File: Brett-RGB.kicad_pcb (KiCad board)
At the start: 2 copper layers, 223 x 71 mm, 182 parts, among them P1 CONN_02X05, P2 USB_OTG, SW1 SW_PUSH, SW10 SW_PUSH, SW11 SW_PUSH, SW12 SW_PUSH, SW13 SW_PUSH, SW14 SW_PUSH, SW15 SW_PUSH, SW16 SW_PUSH, SW17 SW_PUSH, SW18 SW_PUSH, SW19 SW_PUSH, SW2 SW_PUSH, SW20 SW_PUSH, SW21 SW_PUSH, SW22 SW_PUSH, SW23 SW_PUSH, SW24 SW_PUSH, SW25 SW_PUSH, SW26 SW_PUSH, SW27 SW_PUSH, SW28 SW_PUSH, SW29 SW_PUSH, SW3 SW_PUSH, SW30 SW_PUSH, SW31 SW_PUSH, SW32 SW_PUSH, SW33 SW_PUSH, SW34 SW_PUSH, SW35 SW_PUSH, SW36 SW_PUSH, SW37 SW_PUSH, SW38 SW_PUSH, SW39 SW_PUSH, SW4 SW_PUSH, SW40 SW_PUSH, SW41 SW_PUSH, SW42 SW_PUSH, SW43 SW_PUSH, SW44 SW_PUSH, SW45 SW_PUSH, SW46 SW_PUSH, SW47 SW_PUSH, SW48 Reset, SW5 SW_PUSH, SW6 SW_PUSH, SW7 SW_PUSH, SW8 SW_PUSH, SW9 SW_PUSH, U1 IS31FL3732, U2 MK20DX256VLH7, X1 CRYSTAL_SMD

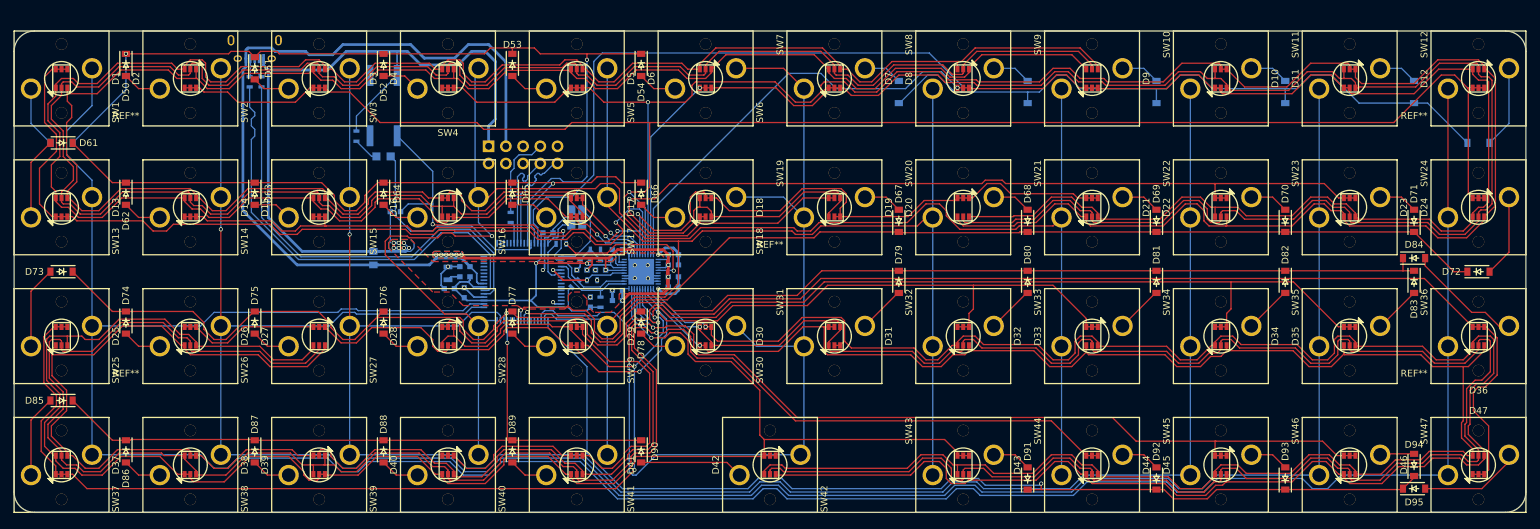
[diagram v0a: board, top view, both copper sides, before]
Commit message: Reworked the Board
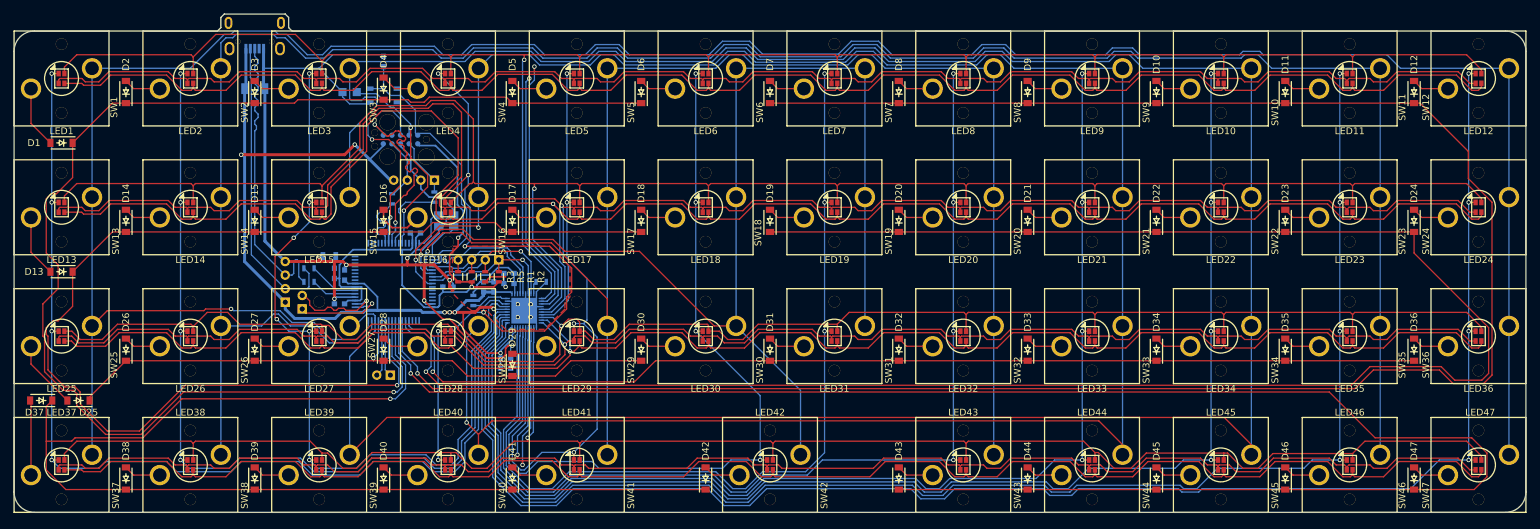
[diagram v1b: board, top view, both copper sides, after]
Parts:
- removed C14, C15, C17, C20, C21: 0.1uF, Capacitors_SMD:C_0603
- removed C18, C19: 1uF, Capacitors_SMD:C_0603
- removed D48: LED, LEDs:LED_0805
- removed D49, D50, D51, D52, D53, D54, D55, D56, D57, D58, D59, D60, D61, D62, D63, D64, D65, D66, D67, D68, D69, D70, D71, D72, D73, D74, D75, D76, D77, D78, D79, D80, D81, D82, D83, D84, D85, D86, D87, D88, D89, D90, D91, D92, D93, D94, D95: D_Small, Diodes_SMD:SOD-123
- added C11: 0.1uF, Capacitors_SMD:C_0603, B.Cu at (97.2, 64.8)
- added LED1: Led_RGB_CA, lib.pretty:RGB-0606, F.Cu at (45.0, 42.0)
- added LED10: Led_RGB_CA, lib.pretty:RGB-0606, F.Cu at (216.0, 42.0)
- added LED11: Led_RGB_CA, lib.pretty:RGB-0606, F.Cu at (235.0, 42.0)
- added LED12: Led_RGB_CA, lib.pretty:RGB-0606, F.Cu at (254.0, 42.0)
- added LED13: Led_RGB_CA, lib.pretty:RGB-0606, F.Cu at (45.0, 61.0)
- added LED14: Led_RGB_CA, lib.pretty:RGB-0606, F.Cu at (64.0, 61.0)
- added LED15: Led_RGB_CA, lib.pretty:RGB-0606, F.Cu at (83.0, 61.0)
- added LED16: Led_RGB_CA, lib.pretty:RGB-0606, F.Cu at (102.0, 61.0)
- added LED17: Led_RGB_CA, lib.pretty:RGB-0606, F.Cu at (121.0, 61.0)
- added LED18: Led_RGB_CA, lib.pretty:RGB-0606, F.Cu at (140.0, 61.0)
- added LED19: Led_RGB_CA, lib.pretty:RGB-0606, F.Cu at (159.0, 61.0)
- added LED2: Led_RGB_CA, lib.pretty:RGB-0606, F.Cu at (64.0, 42.0)
- added LED20: Led_RGB_CA, lib.pretty:RGB-0606, F.Cu at (178.0, 61.0)
- added LED21: Led_RGB_CA, lib.pretty:RGB-0606, F.Cu at (197.0, 61.0)
- added LED22: Led_RGB_CA, lib.pretty:RGB-0606, F.Cu at (216.0, 61.0)
- added LED23: Led_RGB_CA, lib.pretty:RGB-0606, F.Cu at (235.0, 61.0)
- added LED24: Led_RGB_CA, lib.pretty:RGB-0606, F.Cu at (254.0, 61.0)
- added LED25: Led_RGB_CA, lib.pretty:RGB-0606, F.Cu at (45.0, 80.0)
- added LED26: Led_RGB_CA, lib.pretty:RGB-0606, F.Cu at (64.0, 80.0)
- added LED27: Led_RGB_CA, lib.pretty:RGB-0606, F.Cu at (83.0, 80.0)
- added LED28: Led_RGB_CA, lib.pretty:RGB-0606, F.Cu at (102.0, 80.0)
- added LED29: Led_RGB_CA, lib.pretty:RGB-0606, F.Cu at (121.0, 80.0)
- added LED3: Led_RGB_CA, lib.pretty:RGB-0606, F.Cu at (83.0, 42.0)
- added LED30: Led_RGB_CA, lib.pretty:RGB-0606, F.Cu at (140.0, 80.0)
- added LED31: Led_RGB_CA, lib.pretty:RGB-0606, F.Cu at (159.0, 80.0)
- added LED32: Led_RGB_CA, lib.pretty:RGB-0606, F.Cu at (178.0, 80.0)
- added LED33: Led_RGB_CA, lib.pretty:RGB-0606, F.Cu at (197.0, 80.0)
- added LED34: Led_RGB_CA, lib.pretty:RGB-0606, F.Cu at (216.0, 80.0)
- added LED35: Led_RGB_CA, lib.pretty:RGB-0606, F.Cu at (235.0, 80.0)
- added LED36: Led_RGB_CA, lib.pretty:RGB-0606, F.Cu at (254.0, 80.0)
- added LED37: Led_RGB_CA, lib.pretty:RGB-0606, F.Cu at (45.0, 99.0)
- added LED38: Led_RGB_CA, lib.pretty:RGB-0606, F.Cu at (64.0, 99.0)
- added LED39: Led_RGB_CA, lib.pretty:RGB-0606, F.Cu at (83.0, 99.0)
- added LED4: Led_RGB_CA, lib.pretty:RGB-0606, F.Cu at (102.0, 42.0)
- added LED40: Led_RGB_CA, lib.pretty:RGB-0606, F.Cu at (102.0, 99.0)
- added LED41: Led_RGB_CA, lib.pretty:RGB-0606, F.Cu at (121.0, 99.0)
- added LED42: Led_RGB_CA, lib.pretty:RGB-0606, F.Cu at (149.5, 99.0)
- added LED43: Led_RGB_CA, lib.pretty:RGB-0606, F.Cu at (178.0, 99.0)
- added LED44: Led_RGB_CA, lib.pretty:RGB-0606, F.Cu at (197.0, 99.0)
- added LED45: Led_RGB_CA, lib.pretty:RGB-0606, F.Cu at (216.0, 99.0)
- added LED46: Led_RGB_CA, lib.pretty:RGB-0606, F.Cu at (235.0, 99.0)
- added LED47: Led_RGB_CA, lib.pretty:RGB-0606, F.Cu at (254.0, 99.0)
- added LED48: LED, lib.pretty:LED_0805, B.Cu at (87.5, 44.0)
- added LED5: Led_RGB_CA, lib.pretty:RGB-0606, F.Cu at (121.0, 42.0)
- added LED6: Led_RGB_CA, lib.pretty:RGB-0606, F.Cu at (140.0, 42.0)
- added LED7: Led_RGB_CA, lib.pretty:RGB-0606, F.Cu at (159.0, 42.0)
- added LED8: Led_RGB_CA, lib.pretty:RGB-0606, F.Cu at (178.0, 42.0)
- added LED9: Led_RGB_CA, lib.pretty:RGB-0606, F.Cu at (197.0, 42.0)
- added P3: CONN_01X04, lib.pretty:Conn-4, B.Cu at (97.0, 57.0)
- added P4: FLASH_HDR, lib.pretty:JLINK_NEEDLE, B.Cu at (95.0, 51.0)
- added P5: CONN_01X04, lib.pretty:Conn-4, B.Cu at (106.5, 68.8)
- added P6: CONN_01X02, lib.pretty:Conn-2, B.Cu at (92.5, 85.8)
- added P7: CONN_01X02, lib.pretty:Conn-2, B.Cu at (80.5, 75.0)
- added R11: 100, Resistors_SMD:R_0603, B.Cu at (100.0, 59.5)
- C1: value 100uF -> 0.1uF; footprint Capacitors_SMD:C_0805 -> Capacitors_SMD:C_0603
- C12: value 100n -> 0.1uF
- C13, C3: value 1uF -> 0.1uF
- C4: value 0.1uF -> 100uF; footprint Capacitors_SMD:C_0603 -> Capacitors_SMD:C_1206
- C5, C7: value 0.1uF -> 1uF
- C9: value 2.2uF -> 0.1uF
- D1, D10, D11, D12, D13, D14, D15, D16, D17, D18, D19, D2, D20, D21, D22, D23, D24, D25, D26, D27, D28, D29, D3, D30, D31, D32, D33, D34, D35, D36, D37, D38, D39, D4, D40, D41, D42, D43, D44, D45, D46, D47, D5, D6, D7, D8, D9: value LED_RGB -> D_Small; footprint mx2a:plcc-6 -> lib.pretty:SOD-123
- P1: value CONN_02X05 -> USB_OTG; footprint Pin_Headers:Pin_Header_Straight_2x05 -> lib.pretty:Micro-USB_629105150521
- P2: value USB_OTG -> CONN_01X04; footprint Connect:USB_Micro-B -> lib.pretty:Conn-4
- R1: value 1k -> 100k; moved to F.Cu
- R2: moved to F.Cu
- R3: value 33 -> 4.7k; moved to F.Cu
- R4: value 33 -> 100k
- R5: value 5M -> 4.7k; footprint Resistors_SMD:R_0805 -> Resistors_SMD:R_0603; moved to F.Cu
- R6: value 20k -> 33
- R7: value 1k -> 33
- R8: value 1k -> 20k
- R9: value 100k -> 5M; footprint Resistors_SMD:R_0603 -> Resistors_SMD:R_0805
- SW1, SW10, SW11, SW12, SW13, SW14, SW15, SW16, SW17, SW18, SW19, SW2, SW20, SW21, SW22, SW23, SW24, SW25, SW26, SW27, SW28, SW29, SW3, SW30, SW31, SW32, SW33, SW34, SW35, SW36, SW37, SW38, SW39, SW4, SW40, SW41, SW42, SW43, SW44, SW45, SW46, SW47, SW5, SW6, SW7, SW8, SW9: footprint mx2a:RomerG -> lib.pretty:RomerG
- SW48: value Reset -> TAC_SWITCH; footprint mx2a:KSEM31GLFS -> lib.pretty:PTS810
- U1: value IS31FL3732 -> IS31FL3737
- U2: value MK20DX256VLH7 -> MK20DX256VLH7-RESCUE-RainbowFox
- moved C4 66.4 mm to (73.5, 43.5)
- moved R4 50.7 mm to (115.8, 72.0), turned to 180 degrees
- moved R6 42.3 mm to (81.5, 70.0), turned to 180 degrees
- moved R3 42.1 mm to (103.5, 71.2), turned to 90 degrees
- moved P1 39.9 mm to (73.5, 32.0), turned to 0 degrees
- moved R7 39.3 mm to (81.5, 72.0), turned to 180 degrees
- moved R9 38.9 mm to (84.5, 68.2)
- moved P2 34.8 mm to (78.0, 72.0), turned to 90 degrees
- moved R1 28.1 mm to (107.5, 71.2)
- moved C5 28.0 mm to (107.2, 72.8), turned to 90 degrees
- moved C3 26.5 mm to (108.8, 72.8), turned to 90 degrees
- moved C13 25.1 mm to (102.0, 72.8), turned to 0 degrees
- moved C2 24.4 mm to (111.0, 72.2), turned to 180 degrees
- moved C12 22.2 mm to (92.5, 39.5), turned to 90 degrees
- moved C1 20.1 mm to (111.0, 70.8), turned to 180 degrees
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- renumbered REF** to ?
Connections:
- net /MCU/X+ renamed Net-(U2-Pad32)
- net /MCU/X- renamed Net-(U2-Pad33)
- C1 pad 1: GND -> +3V3
- C1 pad 2: +5V -> GND
- C10 pad 1: GND -> +5V
- C10 pad 2: +5V -> GND
- C13 pad 1: +5V -> +3V3
- C2 pad 1: +5V -> +3V3
- C6 pad 1: +3V3 -> +5V
- C7 pad 1: +3V3 -> +5V
- C8 pad 2: GND -> Net-(C8-Pad2)
- C9 pad 1: Net-(C9-Pad1) -> +3V3
- C9 pad 2: +3V3 -> GND
- D1 pad 1: /MCU/A1 -> /MCU/PTD0
- D1 pad 2: /MCU/A2 -> Net-(D1-Pad2)
- D10 pad 1: /MCU/A9 -> /MCU/PTC9
- D10 pad 2: /MCU/A9 -> Net-(D10-Pad2)
- D11 pad 1: /MCU/A7 -> /MCU/PTC9
- D11 pad 2: /MCU/A7 -> Net-(D11-Pad2)
- D12 pad 1: /MCU/A7 -> /MCU/PTC9
- D12 pad 2: /MCU/A8 -> Net-(D12-Pad2)
- D13 pad 1: /MCU/A5 -> /MCU/PTD1
- D13 pad 2: /MCU/A5 -> Net-(D13-Pad2)
- D14 pad 1: /MCU/A4 -> /MCU/PTD1
- D14 pad 2: /MCU/A4 -> Net-(D14-Pad2)
- D15 pad 1: /MCU/A3 -> /MCU/PTD1
- D15 pad 2: /MCU/A2 -> Net-(D15-Pad2)
- D16 pad 1: /MCU/A2 -> /MCU/PTD1
- D16 pad 2: /MCU/A3 -> Net-(D16-Pad2)
- D17 pad 1: /MCU/A1 -> /MCU/PTD1
- D17 pad 2: /MCU/A1 -> Net-(D17-Pad2)
- D18 pad 1: /MCU/A6 -> /MCU/PTD1
- D18 pad 2: /MCU/A6 -> Net-(D18-Pad2)
- D19 pad 1: /MCU/A5 -> /MCU/PTC8
- D19 pad 2: /MCU/A4 -> Net-(D19-Pad2)
- D2 pad 1: /MCU/A3 -> /MCU/PTD0
- D2 pad 2: /MCU/A2 -> Net-(D2-Pad2)
- D20 pad 1: /MCU/A4 -> /MCU/PTC8
- D20 pad 2: /MCU/A4 -> Net-(D20-Pad2)
- D21 pad 1: /MCU/A7 -> /MCU/PTC8
- D21 pad 2: /MCU/A8 -> Net-(D21-Pad2)
- D22 pad 1: /MCU/A5 -> /MCU/PTC8
- D22 pad 2: /MCU/A5 -> Net-(D22-Pad2)
- D23 pad 1: /MCU/A7 -> /MCU/PTC8
- D23 pad 2: /MCU/A8 -> Net-(D23-Pad2)
- D24 pad 1: /MCU/A6 -> /MCU/PTC8
- D24 pad 2: /MCU/A6 -> Net-(D24-Pad2)
- D25 pad 1: /MCU/B7 -> /MCU/PTD4
- D25 pad 2: /MCU/B8 -> Net-(D25-Pad2)
- D26 pad 1: /MCU/B7 -> /MCU/PTD4
- D26 pad 2: /MCU/B8 -> Net-(D26-Pad2)
- D27 pad 1: /MCU/B4 -> /MCU/PTD4
- D27 pad 2: /MCU/B4 -> Net-(D27-Pad2)
- D28 pad 1: /MCU/B5 -> /MCU/PTD4
- D28 pad 2: /MCU/B6 -> Net-(D28-Pad2)
- D29 pad 1: /MCU/B4 -> /MCU/PTD4
- D29 pad 2: /MCU/B4 -> Net-(D29-Pad2)
- D3 pad 1: /MCU/A6 -> /MCU/PTD0
- D3 pad 2: /MCU/A6 -> Net-(D3-Pad2)
- D30 pad 1: /MCU/B3 -> /MCU/PTD4
- D30 pad 2: /MCU/B3 -> Net-(D30-Pad2)
- D31 pad 1: /MCU/B2 -> /MCU/PTC7
- D31 pad 2: /MCU/B1 -> Net-(D31-Pad2)
- D32 pad 1: /MCU/B1 -> /MCU/PTC7
- D32 pad 2: /MCU/B2 -> Net-(D32-Pad2)
- D33 pad 1: /MCU/B4 -> /MCU/PTC7
- D33 pad 2: /MCU/B4 -> Net-(D33-Pad2)
- D34 pad 1: /MCU/B1 -> /MCU/PTC7
- D34 pad 2: /MCU/B2 -> Net-(D34-Pad2)
- D35 pad 1: /MCU/B5 -> /MCU/PTC7
- D35 pad 2: /MCU/B5 -> Net-(D35-Pad2)
- D36 pad 1: /MCU/B1 -> /MCU/PTC7
- D36 pad 2: /MCU/B2 -> Net-(D36-Pad2)
- D37 pad 1: /MCU/B5 -> /MCU/PTC11
- D37 pad 2: /MCU/B5 -> Net-(D37-Pad2)
- D38 pad 1: /MCU/B9 -> /MCU/PTC11
- D38 pad 2: /MCU/B9 -> Net-(D38-Pad2)
- D39 pad 1: /MCU/B8 -> /MCU/PTC11
- D39 pad 2: /MCU/B7 -> Net-(D39-Pad2)
- D4 pad 1: /MCU/A3 -> /MCU/PTD0
- D4 pad 2: /MCU/A2 -> Net-(D4-Pad2)
- D40 pad 1: /MCU/B6 -> /MCU/PTC11
- D40 pad 2: /MCU/B6 -> Net-(D40-Pad2)
- D41 pad 1: /MCU/B9 -> /MCU/PTC11
- D41 pad 2: /MCU/B8 -> Net-(D41-Pad2)
- D42 pad 1: /MCU/B9 -> /MCU/PTC11
- D42 pad 2: /MCU/B9 -> Net-(D42-Pad2)
- D43 pad 1: /MCU/B3 -> /MCU/PTC10
- D43 pad 2: /MCU/B2 -> Net-(D43-Pad2)
- D44 pad 1: /MCU/B1 -> /MCU/PTC10
- D44 pad 2: /MCU/B2 -> Net-(D44-Pad2)
- D45 pad 1: /MCU/B7 -> /MCU/PTC10
- D45 pad 2: /MCU/B7 -> Net-(D45-Pad2)
- D46 pad 1: /MCU/B1 -> /MCU/PTC10
- D46 pad 2: /MCU/B2 -> Net-(D46-Pad2)
- D47 pad 1: /MCU/B6 -> /MCU/PTC10
- D47 pad 2: /MCU/B6 -> Net-(D47-Pad2)
- D5 pad 1: /MCU/A7 -> /MCU/PTD0
- D5 pad 2: /MCU/A7 -> Net-(D5-Pad2)
- D6 pad 1: /MCU/A3 -> /MCU/PTD0
- D6 pad 2: /MCU/A2 -> Net-(D6-Pad2)
- D7 pad 1: /MCU/A8 -> /MCU/PTC9
- D7 pad 2: /MCU/A8 -> Net-(D7-Pad2)
- D8 pad 1: /MCU/A3 -> /MCU/PTC9
- D8 pad 2: /MCU/A2 -> Net-(D8-Pad2)
- D9 pad 1: /MCU/A9 -> /MCU/PTC9
- D9 pad 2: /MCU/A9 -> Net-(D9-Pad2)
- P1 pad 1: GND -> +5V
- P1 pad 2: (no net) -> /MCU/USB_D-
- P1 pad 3: +5V -> /MCU/USB_D+
- P1 pad 5: (no net) -> GND
- P2 pad 2: Net-(P2-Pad2) -> /MCU/USB_D-
- P2 pad 3: Net-(P2-Pad3) -> /MCU/USB_D+
- P2 pad 4: (no net) -> GND
- R1 pad 1: Net-(D48-Pad1) -> GND
- R1 pad 2: GND -> /MCU/SDB
- R10 pad 1: /MCU/SWD_CLK -> Net-(R10-Pad1)
- R10 pad 2: Net-(R10-Pad2) -> /MCU/SWD_CLK
- R2 pad 1: /MCU/INTB -> +3V3
- R2 pad 2: Net-(R2-Pad2) -> /MCU/INTB
- R3 pad 1: Net-(P2-Pad2) -> +3V3
- R3 pad 2: /MCU/D- -> /MCU/SCL
- R4 pad 1: Net-(P2-Pad3) -> GND
- R4 pad 2: /MCU/D+ -> Net-(R4-Pad2)
- R5 pad 1: Net-(C9-Pad1) -> +3V3
- R5 pad 2: GND -> /MCU/SDA
- R6 pad 1: GND -> /MCU/D-
- R6 pad 2: /MCU/R_Ext -> /MCU/USB_D-
- R7 pad 1: /MCU/SCL -> /MCU/D+
- R7 pad 2: +3V3 -> /MCU/USB_D+
- R8 pad 1: /MCU/SDA -> Net-(R8-Pad1)
- R8 pad 2: +3V3 -> GND
- R9 pad 1: GND -> Net-(C8-Pad2)
- R9 pad 2: /MCU/SDB -> GND
- SW1 pad 1: Net-(D49-Pad2) -> Net-(D1-Pad2)
- SW1 pad 2: /MCU/Col1 -> /MCU/PTD7
- SW10 pad 1: Net-(D58-Pad2) -> Net-(D10-Pad2)
- SW10 pad 2: /MCU/Col3 -> /MCU/PTD5
- SW11 pad 1: Net-(D59-Pad2) -> Net-(D11-Pad2)
- SW11 pad 2: /MCU/Col2 -> /MCU/PTD6
- SW12 pad 1: Net-(D60-Pad2) -> Net-(D12-Pad2)
- SW12 pad 2: /MCU/Col1 -> /MCU/PTD7
- SW13 pad 1: Net-(D61-Pad2) -> Net-(D13-Pad2)
- SW13 pad 2: /MCU/Col1 -> /MCU/PTD7
- SW14 pad 1: Net-(D62-Pad2) -> Net-(D14-Pad2)
- SW14 pad 2: /MCU/Col2 -> /MCU/PTD6
- SW15 pad 1: Net-(D63-Pad2) -> Net-(D15-Pad2)
- SW15 pad 2: /MCU/Col3 -> /MCU/PTD5
- SW16 pad 1: Net-(D64-Pad2) -> Net-(D16-Pad2)
- SW16 pad 2: /MCU/Col4 -> /MCU/PTB18
- SW17 pad 1: Net-(D65-Pad2) -> Net-(D17-Pad2)
- SW17 pad 2: /MCU/Col5 -> /MCU/PTB2
- SW18 pad 1: Net-(D66-Pad2) -> Net-(D18-Pad2)
- SW18 pad 2: /MCU/Col6 -> /MCU/PTB3
- SW19 pad 1: Net-(D67-Pad2) -> Net-(D19-Pad2)
- SW19 pad 2: /MCU/Col6 -> /MCU/PTB3
- SW2 pad 1: Net-(D50-Pad2) -> Net-(D2-Pad2)
- SW2 pad 2: /MCU/Col2 -> /MCU/PTD6
- SW20 pad 1: Net-(D68-Pad2) -> Net-(D20-Pad2)
- SW20 pad 2: /MCU/Col5 -> /MCU/PTB2
- SW21 pad 1: Net-(D69-Pad2) -> Net-(D21-Pad2)
- SW21 pad 2: /MCU/Col4 -> /MCU/PTB18
- SW22 pad 1: Net-(D70-Pad2) -> Net-(D22-Pad2)
- SW22 pad 2: /MCU/Col3 -> /MCU/PTD5
- SW23 pad 1: Net-(D71-Pad2) -> Net-(D23-Pad2)
- SW23 pad 2: /MCU/Col2 -> /MCU/PTD6
- SW24 pad 1: Net-(D72-Pad2) -> Net-(D24-Pad2)
- SW24 pad 2: /MCU/Col1 -> /MCU/PTD7
- SW25 pad 1: Net-(D73-Pad2) -> Net-(D25-Pad2)
- SW25 pad 2: /MCU/Col1 -> /MCU/PTD7
- SW26 pad 1: Net-(D74-Pad2) -> Net-(D26-Pad2)
- SW26 pad 2: /MCU/Col2 -> /MCU/PTD6
- SW27 pad 1: Net-(D75-Pad2) -> Net-(D27-Pad2)
- SW27 pad 2: /MCU/Col3 -> /MCU/PTD5
- SW28 pad 1: Net-(D76-Pad2) -> Net-(D28-Pad2)
- SW28 pad 2: /MCU/Col4 -> /MCU/PTB18
- SW29 pad 1: Net-(D77-Pad2) -> Net-(D29-Pad2)
- SW29 pad 2: /MCU/Col5 -> /MCU/PTB2
- SW3 pad 1: Net-(D51-Pad2) -> Net-(D3-Pad2)
- SW3 pad 2: /MCU/Col3 -> /MCU/PTD5
- SW30 pad 1: Net-(D78-Pad2) -> Net-(D30-Pad2)
- SW30 pad 2: /MCU/Col6 -> /MCU/PTB3
- SW31 pad 1: Net-(D79-Pad2) -> Net-(D31-Pad2)
- SW31 pad 2: /MCU/Col6 -> /MCU/PTB3
- SW32 pad 1: Net-(D80-Pad2) -> Net-(D32-Pad2)
- SW32 pad 2: /MCU/Col5 -> /MCU/PTB2
- SW33 pad 1: Net-(D81-Pad2) -> Net-(D33-Pad2)
- SW33 pad 2: /MCU/Col4 -> /MCU/PTB18
- SW34 pad 1: Net-(D82-Pad2) -> Net-(D34-Pad2)
- SW34 pad 2: /MCU/Col3 -> /MCU/PTD5
- SW35 pad 1: Net-(D83-Pad2) -> Net-(D35-Pad2)
- SW35 pad 2: /MCU/Col2 -> /MCU/PTD6
- SW36 pad 1: Net-(D84-Pad2) -> Net-(D36-Pad2)
- SW36 pad 2: /MCU/Col1 -> /MCU/PTD7
- SW37 pad 1: Net-(D85-Pad2) -> Net-(D37-Pad2)
- SW37 pad 2: /MCU/Col1 -> /MCU/PTD7
- SW38 pad 1: Net-(D86-Pad2) -> Net-(D38-Pad2)
- SW38 pad 2: /MCU/Col2 -> /MCU/PTD6
- SW39 pad 1: Net-(D87-Pad2) -> Net-(D39-Pad2)
- SW39 pad 2: /MCU/Col3 -> /MCU/PTD5
- SW4 pad 1: Net-(D52-Pad2) -> Net-(D4-Pad2)
- SW4 pad 2: /MCU/Col4 -> /MCU/PTB18
- SW40 pad 1: Net-(D88-Pad2) -> Net-(D40-Pad2)
- SW40 pad 2: /MCU/Col4 -> /MCU/PTB18
- SW41 pad 1: Net-(D89-Pad2) -> Net-(D41-Pad2)
- SW41 pad 2: /MCU/Col5 -> /MCU/PTB2
- SW42 pad 1: Net-(D90-Pad2) -> Net-(D42-Pad2)
- SW42 pad 2: /MCU/Col6 -> /MCU/PTB3
- SW43 pad 1: Net-(D91-Pad2) -> Net-(D43-Pad2)
- SW43 pad 2: /MCU/Col5 -> /MCU/PTB2
- SW44 pad 1: Net-(D92-Pad2) -> Net-(D44-Pad2)
- SW44 pad 2: /MCU/Col4 -> /MCU/PTB18
- SW45 pad 1: Net-(D93-Pad2) -> Net-(D45-Pad2)
- SW45 pad 2: /MCU/Col3 -> /MCU/PTD5
- SW46 pad 1: Net-(D94-Pad2) -> Net-(D46-Pad2)
- SW46 pad 2: /MCU/Col2 -> /MCU/PTD6
- SW47 pad 1: Net-(D95-Pad2) -> Net-(D47-Pad2)
- SW47 pad 2: /MCU/Col1 -> /MCU/PTD7
- SW48 pad 1: /MCU/MCU_RESET -> (no net)
- SW48 pad 2: GND -> /MCU/MCU_RESET
- SW48 pad 4: (no net) -> GND
- SW5 pad 1: Net-(D53-Pad2) -> Net-(D5-Pad2)
- SW5 pad 2: /MCU/Col5 -> /MCU/PTB2
- SW6 pad 1: Net-(D54-Pad2) -> Net-(D6-Pad2)
- SW6 pad 2: /MCU/Col6 -> /MCU/PTB3
- SW7 pad 1: Net-(D55-Pad2) -> Net-(D7-Pad2)
- SW7 pad 2: /MCU/Col6 -> /MCU/PTB3
- SW8 pad 1: Net-(D56-Pad2) -> Net-(D8-Pad2)
- SW8 pad 2: /MCU/Col5 -> /MCU/PTB2
- SW9 pad 1: Net-(D57-Pad2) -> Net-(D9-Pad2)
- SW9 pad 2: /MCU/Col4 -> /MCU/PTB18
- U1 pad 1: +5V -> /MCU/SW1
- U1 pad 10: (no net) -> /MCU/SW9
- U1 pad 11: /MCU/B1 -> GND
- U1 pad 12: /MCU/B2 -> /MCU/SW10
- U1 pad 13: /MCU/B3 -> /MCU/SW11
- U1 pad 14: /MCU/B4 -> /MCU/SW12
- U1 pad 15: /MCU/B5 -> /MCU/CS1
- U1 pad 16: /MCU/B6 -> /MCU/CS2
- U1 pad 17: /MCU/B7 -> /MCU/CS3
- U1 pad 18: /MCU/B8 -> /MCU/CS4
- U1 pad 19: /MCU/B9 -> +5V
- U1 pad 2: (no net) -> /MCU/SW2
- U1 pad 20: +5V -> /MCU/CS5
- U1 pad 21: /MCU/SDA -> /MCU/CS6
- U1 pad 22: /MCU/SCL -> /MCU/CS7
- U1 pad 23: GND -> /MCU/CS8
- U1 pad 24: GND -> /MCU/CS9
- U1 pad 25: /MCU/SDB -> /MCU/CS10
- U1 pad 27: +3V3 -> /MCU/CS11
- U1 pad 28: /MCU/R_Ext -> /MCU/CS12
- U1 pad 29: /MCU/C_Filt -> GND
- U1 pad 3: (no net) -> /MCU/SW3
- U1 pad 30: (no net) -> Net-(R8-Pad1)
- U1 pad 31: GND -> +5V
- U1 pad 32: /MCU/A1 -> +3V3
- U1 pad 33: /MCU/A2 -> (no net)
- U1 pad 34: /MCU/A3 -> /MCU/SDA
- U1 pad 35: /MCU/A4 -> /MCU/SCL
- U1 pad 36: /MCU/A5 -> GND
- U1 pad 37: /MCU/A6 -> /MCU/INTB
- U1 pad 38: /MCU/A7 -> /MCU/SDB
- U1 pad 39: /MCU/A8 -> Net-(R4-Pad2)
- U1 pad 4: +5V -> GND
- U1 pad 40: /MCU/A9 -> GND
- U1 pad 5: Net-(R2-Pad2) -> /MCU/SW4
- U1 pad 6: (no net) -> /MCU/SW5
- U1 pad 7: GND -> /MCU/SW6
- U1 pad 8: GND -> /MCU/SW7
- U1 pad 9: GND -> /MCU/SW8
- U2 pad 1: /MCU/Col2 -> /MCU/RX1
- U2 pad 2: /MCU/Col1 -> /MCU/TX1
- U2 pad 22: Net-(R10-Pad2) -> Net-(R10-Pad1)
- U2 pad 25: (no net) -> Net-(R11-Pad1)
- U2 pad 26: /MCU/Row1 -> (no net)
- U2 pad 28: /MCU/Row2 -> (no net)
- U2 pad 29: /MCU/Row5 -> (no net)
- U2 pad 37: /MCU/SDB -> /MCU/PTB2
- U2 pad 38: /MCU/INTB -> /MCU/PTB3
- U2 pad 39: (no net) -> /MCU/SDB
- U2 pad 40: (no net) -> /MCU/INTB
- U2 pad 41: (no net) -> /MCU/PTB18
- U2 pad 49: /MCU/Row8 -> (no net)
- U2 pad 50: /MCU/Col5 -> (no net)
- U2 pad 51: /MCU/Col6 -> (no net)
- U2 pad 52: (no net) -> /MCU/PTC7
- U2 pad 53: (no net) -> /MCU/PTC8
- U2 pad 54: (no net) -> /MCU/PTC9
- U2 pad 55: (no net) -> /MCU/PTC10
- U2 pad 56: /MCU/Row7 -> /MCU/PTC11
- U2 pad 57: /MCU/Row6 -> /MCU/PTD0
- U2 pad 58: (no net) -> /MCU/PTD1
- U2 pad 59: (no net) -> /MCU/RX2
- U2 pad 60: (no net) -> /MCU/TX2
- U2 pad 61: /MCU/Row4 -> /MCU/PTD4
- U2 pad 62: /MCU/Row3 -> /MCU/PTD5
- U2 pad 63: /MCU/Col3 -> /MCU/PTD6
- U2 pad 64: /MCU/Col4 -> /MCU/PTD7
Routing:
- net /MCU/Col1: track 389.3 -> 0.00 mm
- net /MCU/PTD5: track 0.00 -> 388.2 mm
- net /MCU/PTD7: track 0.00 -> 382.2 mm, vias 0 -> 1
- net /MCU/PTD6: track 0.00 -> 327.4 mm
- net /MCU/Col2: track 326.1 -> 0.00 mm, vias 1 -> 0
- net /MCU/PTB18: track 0.00 -> 319.1 mm, vias 0 -> 3
- net /MCU/B7: track 314.2 -> 0.00 mm, vias 1 -> 0
- net /MCU/A7: track 312.9 -> 0.00 mm, vias 1 -> 0
- net /MCU/PTC9: track 0.00 -> 311.0 mm, vias 0 -> 1
- net /MCU/A2: track 306.7 -> 0.00 mm, vias 1 -> 0
- net /MCU/A1: track 301.2 -> 0.00 mm, vias 1 -> 0
- net /MCU/B5: track 299.7 -> 0.00 mm, vias 3 -> 0
- net /MCU/B2: track 299.3 -> 0.00 mm, vias 1 -> 0
- net /MCU/A3: track 294.2 -> 0.00 mm, vias 1 -> 0
- net /MCU/B1: track 293.3 -> 0.00 mm, vias 1 -> 0
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- removed copper zone on B.Cu, net +5V
- removed copper zone on F.Cu, net +5V
- removed copper zone on B.Cu, net GND
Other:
- board size 223 x 71 mm -> 223 x 73.5 mm
- net class Default: via_dia 0.6 -> 0.65
